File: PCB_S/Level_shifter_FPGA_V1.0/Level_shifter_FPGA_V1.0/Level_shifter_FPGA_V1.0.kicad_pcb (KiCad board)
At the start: 6 copper layers, 85 x 85 mm, 185 parts, among them J1 Conn_02x08_Odd_Even, J2 Conn_02x20_Odd_Even, J3 Conn_02x05_Odd_Even, J4 Conn_02x03_Odd_Even, J5 Conn_01x02_Pin, J6 Conn_01x02_Pin, J7 Conn_01x02_Pin, J8 Conn_02x08_Odd_Even, Q1 2N7002, Q10 2N7002, Q11 2N7002, Q12 2N7002, Q13 2N7002, Q14 2N7002, Q15 2N7002, Q16 2N7002, Q17 2N7002, Q18 2N7002, Q19 2N7002, Q2 2N7002, Q20 2N7002, Q21 2N7002, Q22 2N7002, Q23 2N7002, Q24 2N7002, Q25 2N7002, Q26 2N7002, Q27 2N7002, Q28 2N7002, Q29 2N7002, Q3 2N7002, Q30 2N7002, Q31 2N7002, Q32 2N7002, Q33 2N7002, Q34 2N7002, Q35 2N7002, Q36 2N7002, Q37 2N7002, Q38 2N7002, Q39 2N7002, Q4 2N7002, Q40 2N7002, Q41 2N7002, Q42 2N7002, Q43 2N7002, Q44 2N7002, Q45 2N7002, Q46 2N7002, Q47 2N7002, Q48 2N7002, Q49 2N7002, Q5 2N7002, Q50 2N7002, Q51 2N7002, Q52 2N7002, Q53 2N7002, Q54 2N7002, Q55 2N7002, Q56 2N7002, Q57 2N7002, Q58 2N7002, Q59 2N7002, Q6 2N7002, Q60 2N7002, Q61 2N7002, Q62 2N7002, Q63 2N7002, Q64 2N7002, Q65 2N7002, Q66 2N7002, Q67 2N7002, Q68 2N7002, Q69 2N7002, Q7 2N7002, Q70 2N7002, Q71 2N7002, Q72 2N7002, Q73 2N7002, Q74 2N7002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

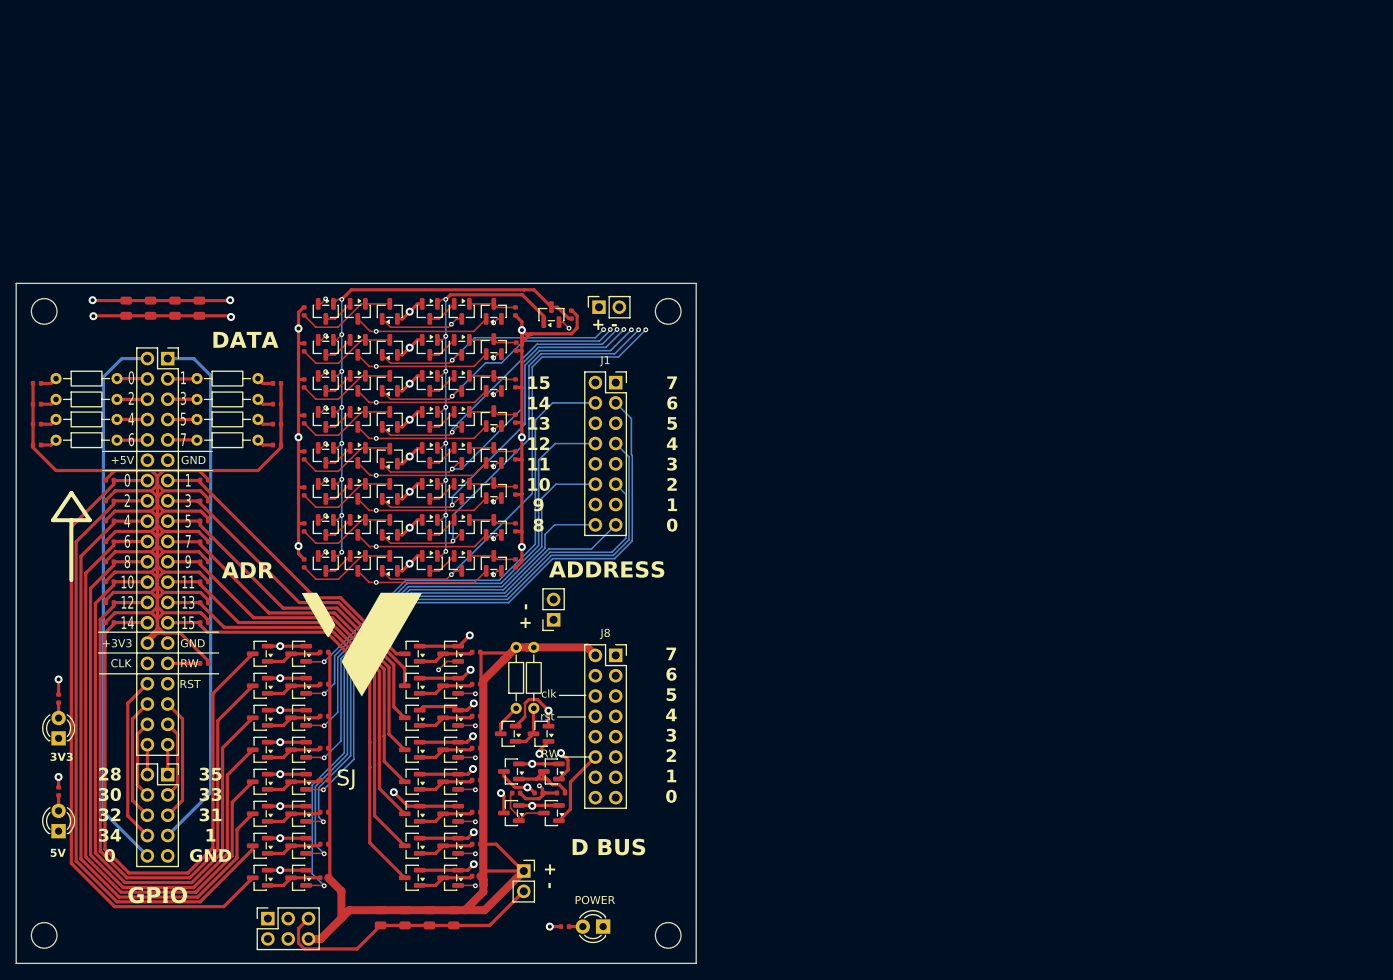
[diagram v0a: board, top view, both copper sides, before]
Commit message: order tomorrow
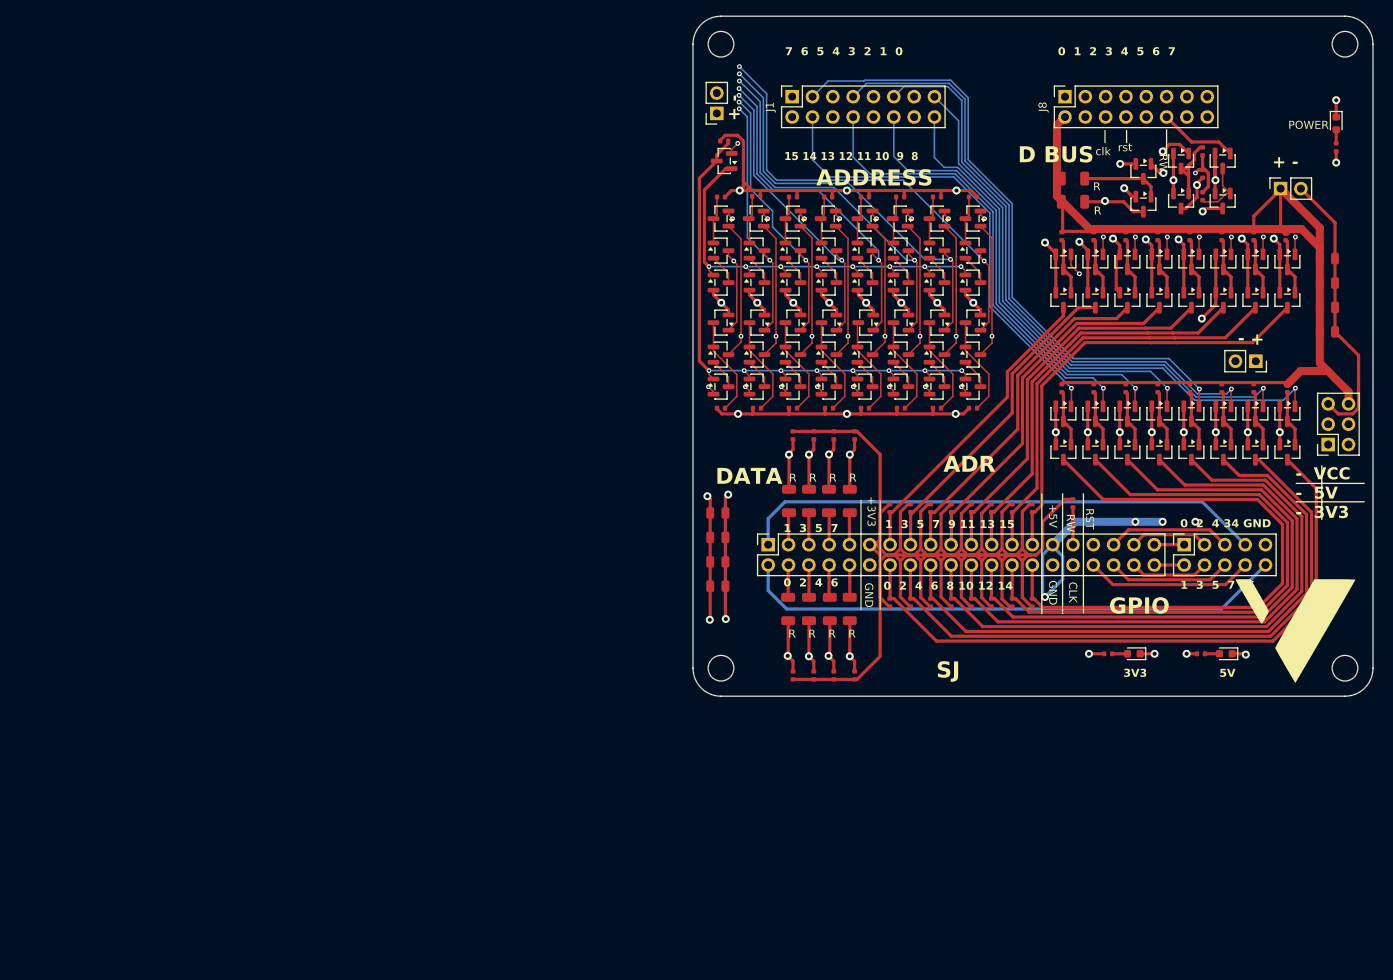
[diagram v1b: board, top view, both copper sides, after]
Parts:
- D1, D2, D3: value LED -> Red; footprint LED_THT:LED_D3.0mm_FlatTop -> PCM_JLCPCB:D_0603
- R1, R2, R22, R24, R3, R4, R5, R6, R7, R8: value R -> 10kΩ; footprint Resistor_THT:R_Axial_DIN0204_L3.6mm_D1.6mm_P7.62mm_Horizontal -> PCM_JLCPCB:R_1206
- moved H25 166.0 mm to (181.5, 111.5), turned to 90 degrees
- moved D3 147.6 mm to (166.6, 109.7), turned to 180 degrees
- moved J4 145.2 mm to (179.4, 83.5), turned to 180 degrees
- moved R74 143.8 mm to (163.5, 109.7), turned to 0 degrees
- moved H25 139.9 mm to (181.5, 33.5), turned to 90 degrees
- moved C8 139.2 mm to (179.3, 69.5), turned to 0 degrees
- moved Q57 139.0 mm to (174.3, 84.5), turned to -90 degrees
- moved C7 138.3 mm to (179.3, 66.4), turned to 0 degrees
- moved C6 137.5 mm to (179.3, 63.4), turned to 0 degrees
- moved R27 137.0 mm to (180.4, 46.4), turned to 90 degrees
- moved C5 136.8 mm to (179.3, 60.3), turned to 0 degrees
- moved Q56 136.5 mm to (174.3, 79.7), turned to -90 degrees
- moved D1 135.9 mm to (180.4, 43.4), turned to -90 degrees
- moved R41 135.1 mm to (174.3, 76.5), turned to -90 degrees
- moved D2 134.8 mm to (155.1, 109.7), turned to 180 degrees
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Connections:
- J2 pad 11: GND -> 3.3V
- J2 pad 12: 5V -> GND
- J2 pad 29: GND -> 5V
- J2 pad 30: 3.3V -> GND
- R2 pad 1: D2 -> Net-(J2-Pin_3)
- R2 pad 2: Net-(J2-Pin_6) -> D1
- R22 pad 1: Net-(Q20-D) -> VCC
- R22 pad 2: VCC -> Net-(Q20-D)
- R24 pad 1: CLK -> VCC
- R24 pad 2: VCC -> CLK
- R3 pad 1: D4 -> D2
- R3 pad 2: Net-(J2-Pin_8) -> Net-(J2-Pin_6)
- R4 pad 1: D6 -> Net-(J2-Pin_5)
- R4 pad 2: Net-(J2-Pin_10) -> D3
- R5 pad 1: Net-(J2-Pin_3) -> D4
- R5 pad 2: D1 -> Net-(J2-Pin_8)
- R6 pad 1: Net-(J2-Pin_5) -> Net-(J2-Pin_7)
- R6 pad 2: D3 -> D5
- R7 pad 1: Net-(J2-Pin_7) -> D6
- R7 pad 2: D5 -> Net-(J2-Pin_10)
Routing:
- net 5V: track 88.9 -> 165.2 mm, vias 1 -> 5
- net 3.3V: track 344.6 -> 383.1 mm
- net D0: track 61.9 -> 67.0 mm, vias 1 -> 2
- net D2: track 60.5 -> 65.1 mm, vias 1 -> 2
- net D6: track 66.8 -> 71.3 mm, vias 1 -> 2
- net D4: track 63.3 -> 67.8 mm, vias 1 -> 2
- net D5: track 38.9 -> 43.3 mm, vias 1 -> 2
- net D1: track 34.8 -> 39.2 mm, vias 1 -> 2
- net D3: track 36.2 -> 40.6 mm, vias 1 -> 2
- net D7: track 45.6 -> 49.8 mm, vias 1 -> 2
- net Net-(Q20-D): track 5.81 -> 9.97 mm
- net CLK: track 14.8 -> 18.7 mm, vias 0 -> 1
- net VCC: track 277.2 -> 275.5 mm
- net RW L: track 55.3 -> 55.9 mm
- net GND: track 222.2 -> 221.8 mm, vias 46 -> 50
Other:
- outline, holes or cut-outs redrawn
- board text added: "- VCC - 5V - 3V3"
- board text added: "0 1 2 3 4 5 6 7"
- board text added: "0 2 4 34 GND"
- board text added: "1 3 5 7 35"
- board text added: "R"
- board text removed: "28 30 32 34 0"
- board text removed: "35 33 31 1 GND"
